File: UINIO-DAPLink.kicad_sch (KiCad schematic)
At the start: 43 parts, among them J1 扩展板串口 & 电源输出, J2 扩展板 JTAG 输出, J3 JTAG_nTRST 跳线选择, J4 3.3V 跳线选择, J5 扩展板 SWD 输入, J6 DAPLink 固件下载接口, J7 SWD 下载输出, U1 ME6211C33M5G, U2 STM32F103C8T6, Y1 8MHz

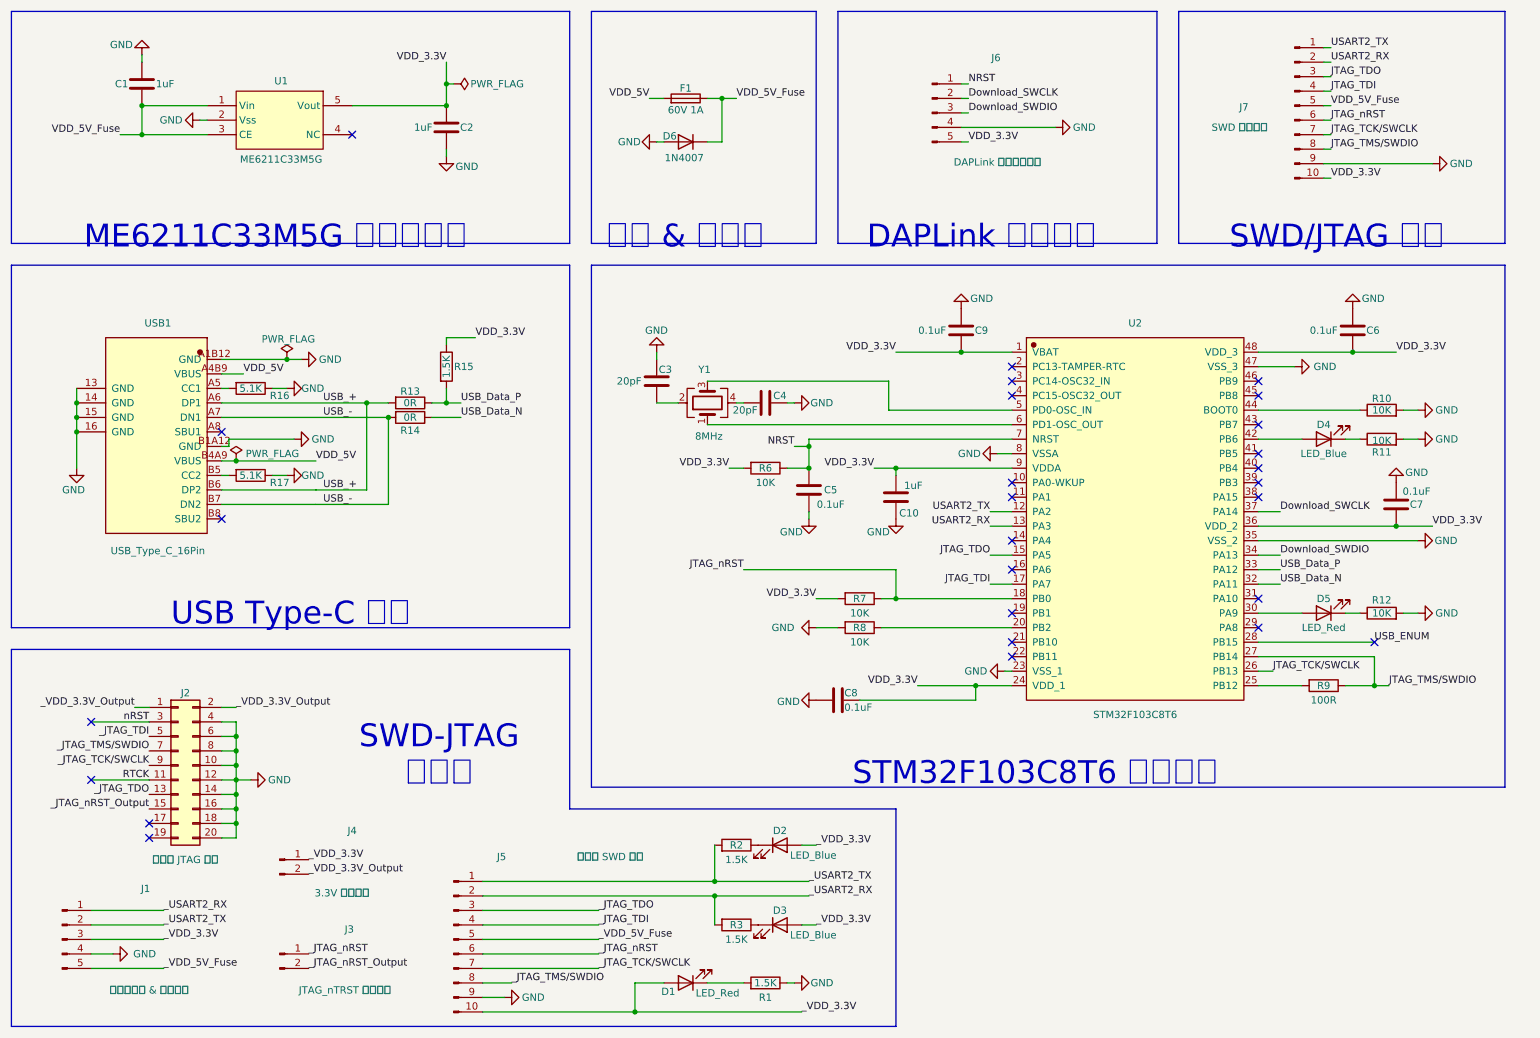
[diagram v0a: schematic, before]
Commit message: Finish PCB Layout.
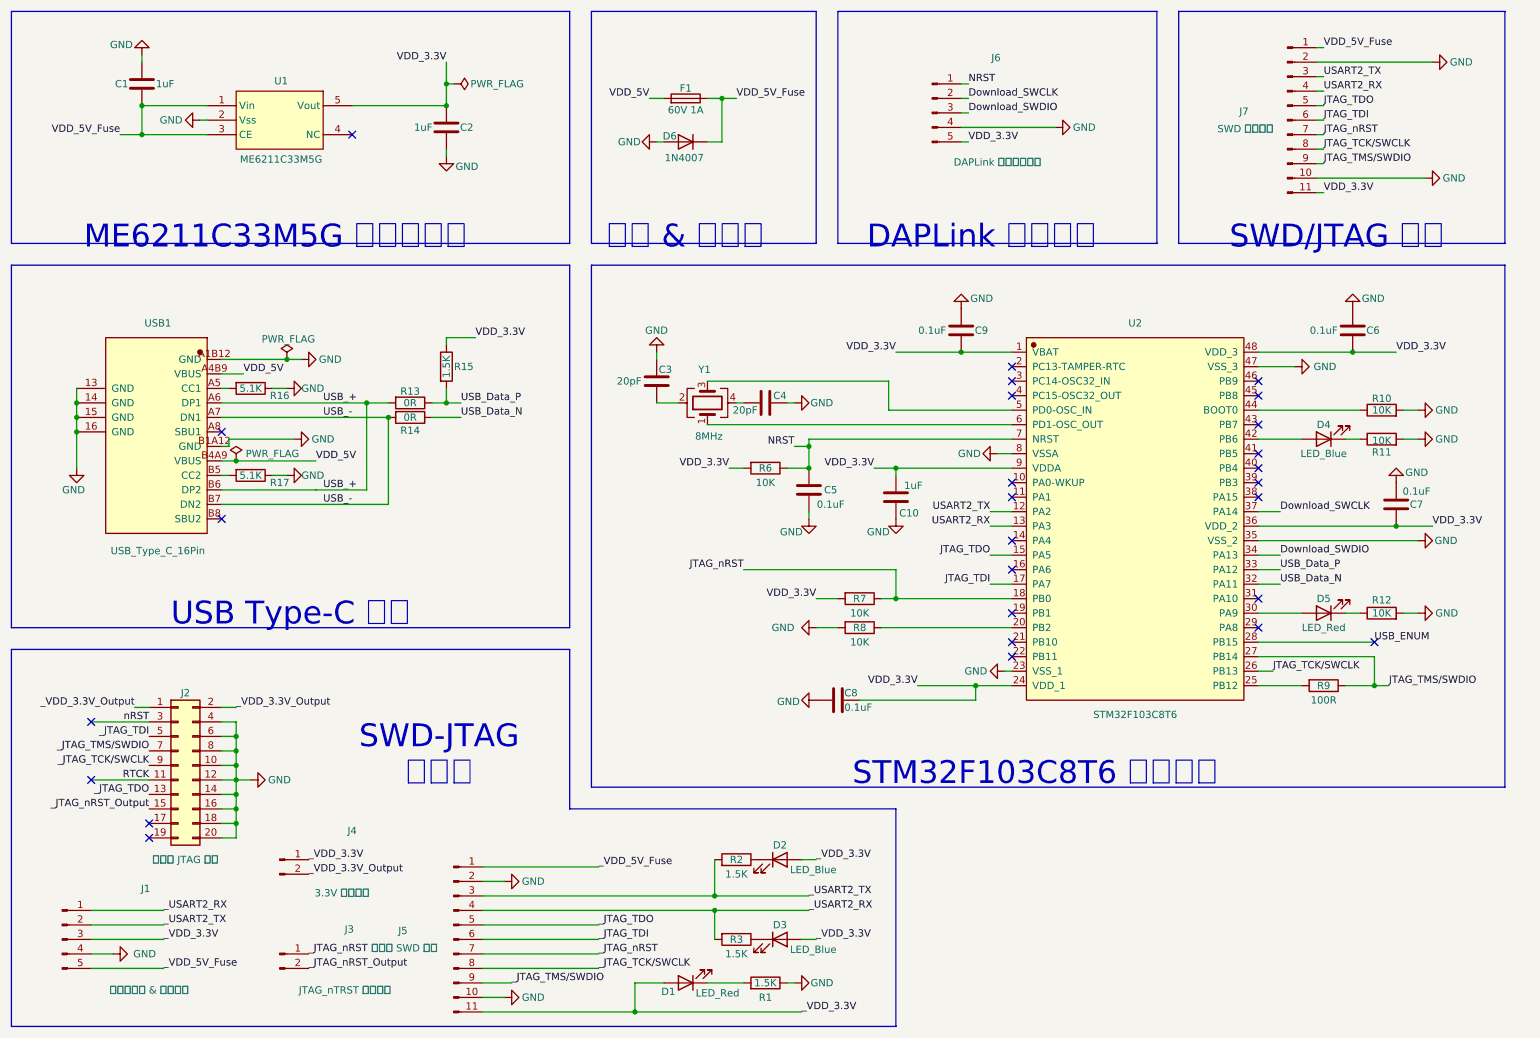
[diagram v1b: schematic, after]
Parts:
- removed J5: 扩展板 SWD 输入, Connector_PinHeader_2.54mm:PinHeader_1x10_P2.54mm_Vertical, symbol Connector:Conn_01x10_Pin
- removed J7: SWD 下载输出, Connector_PinHeader_2.54mm:PinHeader_1x10_P2.54mm_Vertical, symbol Connector:Conn_01x10_Pin
- added J5: 扩展板 SWD 输入, Connector_PinSocket_2.54mm:PinSocket_1x11_P2.54mm_Vertical, symbol Connector:Conn_01x11_Pin
- added J7: SWD 下载输出, Connector_PinSocket_2.54mm:PinSocket_1x11_P2.54mm_Vertical, symbol Connector:Conn_01x11_Pin
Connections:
- net GND: now also J5.10 (Pin_10), J5.2 (Pin_2), J7.10 (Pin_10), J7.2 (Pin_2)
- net JTAG_TCK/SWCLK: now also J7.8 (Pin_8)
- net JTAG_TDI: now also J7.6 (Pin_6)
- net JTAG_TDO: now also J7.5 (Pin_5)
- net JTAG_TMS/SWDIO: now also J7.9 (Pin_9)
- net JTAG_nRST: now also J7.7 (Pin_7)
- net USART2_RX: now also J7.4 (Pin_4)
- net USART2_TX: now also J7.3 (Pin_3)
- net VDD_3.3V: now also J7.11 (Pin_11)
- net VDD_5V_Fuse: now also J7.1 (Pin_1)
- net _JTAG_TCK/SWCLK: now also J5.8 (Pin_8)
- net _JTAG_TDI: now also J5.6 (Pin_6)
- net _JTAG_TDO: now also J5.5 (Pin_5)
- net _JTAG_TMS/SWDIO: now also J5.9 (Pin_9)
- net _JTAG_nRST: now also J5.7 (Pin_7)
- net _USART2_RX: now also J5.4 (Pin_4)
- net _USART2_TX: now also J5.3 (Pin_3)
- net _VDD_3.3V: now also J5.11 (Pin_11)
- net _VDD_5V_Fuse: now also J5.1 (Pin_1)
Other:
- moved on the sheet: D2, D3, R2, R3
